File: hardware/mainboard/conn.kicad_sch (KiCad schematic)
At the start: 25 parts

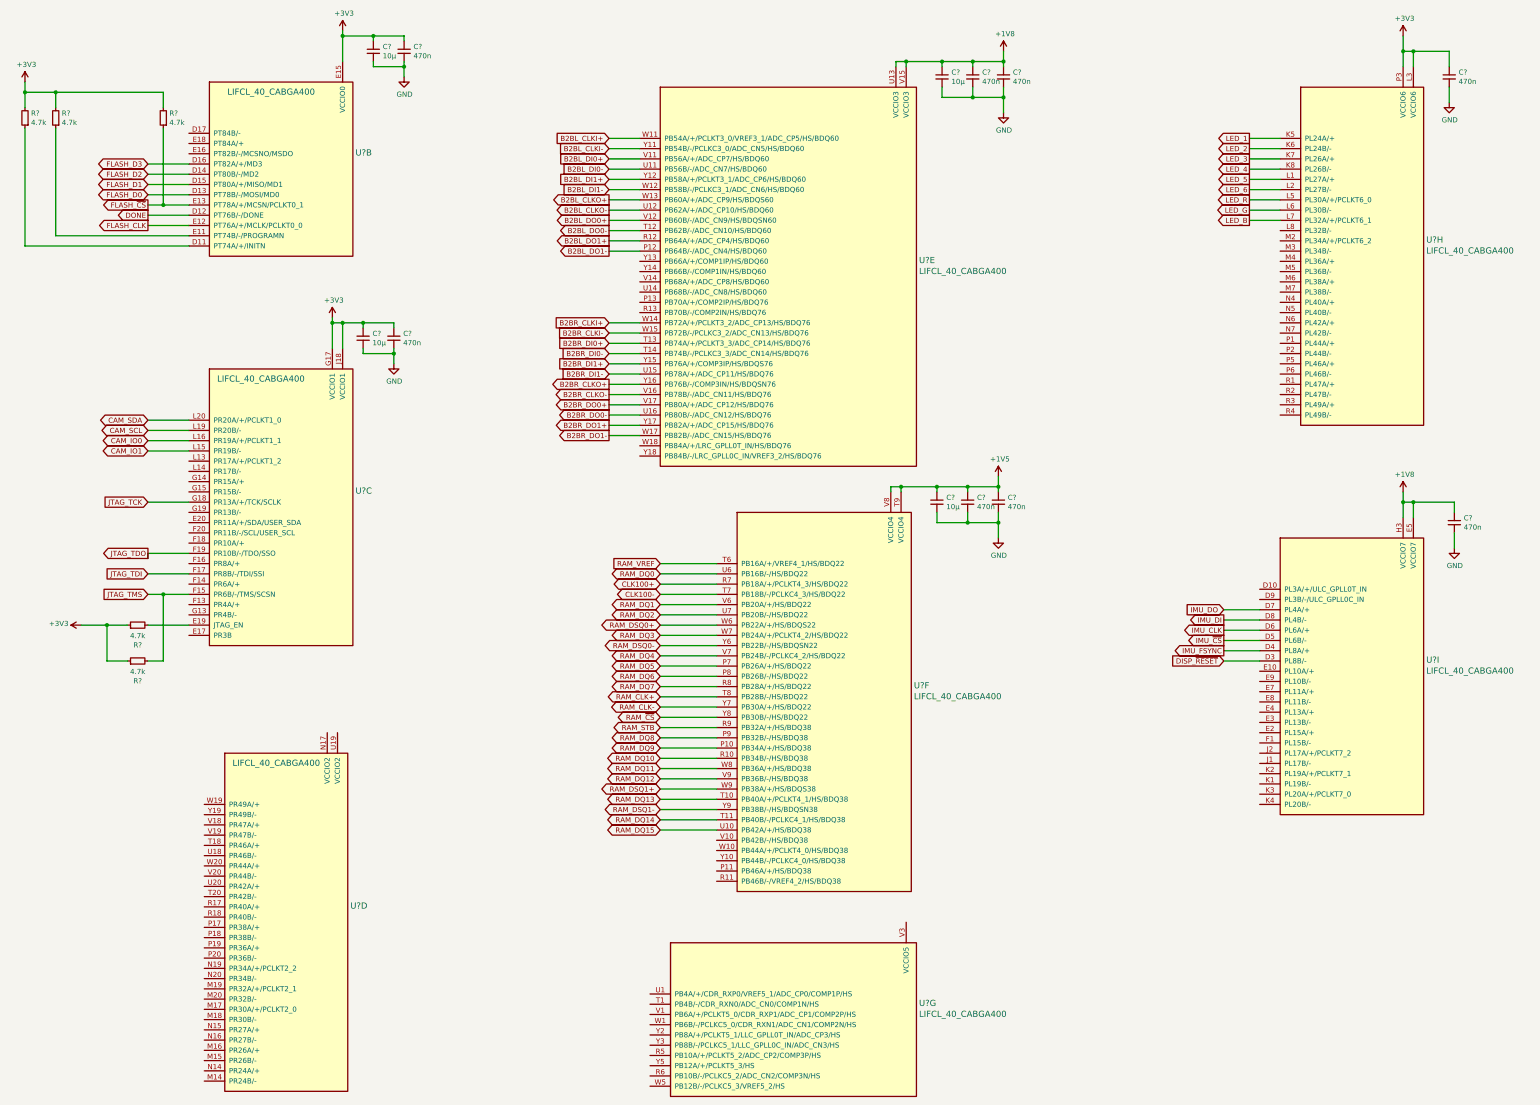
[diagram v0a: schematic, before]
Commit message: Connecting up various bits
Signed-off-by: David Shah <dave@ds0.me>
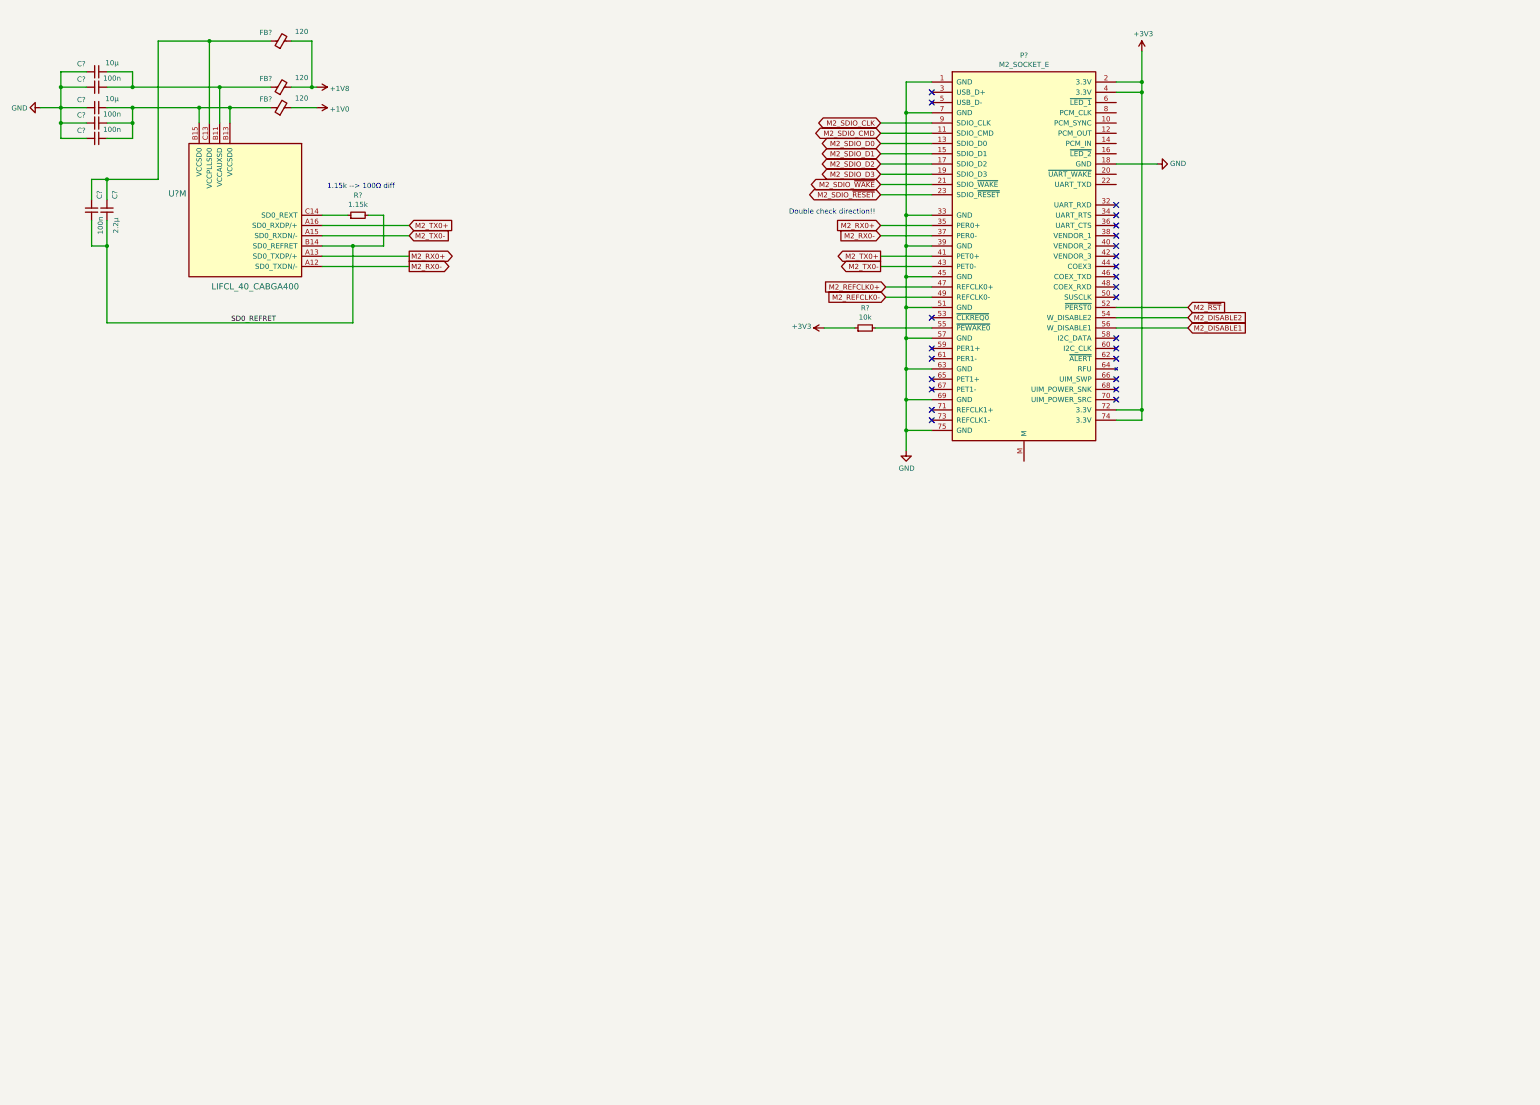
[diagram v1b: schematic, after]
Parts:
- removed C? (x4): 10µ, symbol Device:C_Small
- removed C? (x8): 470n, symbol Device:C_Small
- removed R? (x5): 4.7k, symbol Device:R_Small
- removed U? (x8): LIFCL_40_CABGA400, symbol meowality:LIFCL_40_CABGA400
- added C? (x4): 100n, symbol Device:C_Small
- added C? (x2): 10µ, symbol Device:C_Small
- added C?: 2.2µ, symbol Device:C_Small
- added FB? (x3): 120, symbol Device:FerriteBead_Small
- added P?: M2_SOCKET_E, symbol meowality:M2_SOCKET_E
- added R?: 1.15k, symbol Device:R_Small
- added R?: 10k, symbol Device:R_Small
- added U?: LIFCL_40_CABGA400, symbol meowality:LIFCL_40_CABGA400
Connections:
- net +1V8: now also FB?.2, FB?.2
- net +3V3: now also P?.2 (3.3V), P?.4 (3.3V), P?.72 (3.3V), P?.74 (3.3V), R?.1
- net GND: now also C?.2, C?.2, C?.2, C?.2, C?.2, P?.1 (GND), P?.18 (GND), P?.33 (GND), P?.39 (GND), P?.45 (GND), P?.51 (GND), P?.57 (GND), P?.63 (GND), P?.69 (GND), P?.7 (GND), P?.75 (GND)
- new net: C?.1, C?.1, C?.1, FB?.1, U?.B13 (VCCSD0), U?.B15 (VCCSD0)
- new net: C?.1, C?.1, FB?.1, U?.B11 (VCCAUXSD)
- new net: C?.2, C?.2, FB?.1, U?.C13 (VCCPLLSD0)
- new net: R?.1, U?.C14 (SD0_REXT)
- new net: P?.55 (~PEWAKE0), R?.2
- new net +1V0: FB?.2
- new net M2_DISABLE1: P?.56 (W_DISABLE1)
- new net M2_DISABLE2: P?.54 (W_DISABLE2)
- new net M2_REFCLK0+: P?.47 (REFCLK0+)
- new net M2_REFCLK0-: P?.49 (REFCLK0-)
- new net M2_RX0+: P?.35 (PER0+), U?.A13 (SD0_TXDP/+)
- new net M2_RX0-: P?.37 (PER0-), U?.A12 (SD0_TXDN/-)
- new net M2_SDIO_CLK: P?.9 (SDIO_CLK)
- new net M2_SDIO_CMD: P?.11 (SDIO_CMD)
- new net M2_SDIO_D0: P?.13 (SDIO_D0)
- new net M2_SDIO_D1: P?.15 (SDIO_D1)
- new net M2_SDIO_D2: P?.17 (SDIO_D2)
- new net M2_SDIO_D3: P?.19 (SDIO_D3)
- new net M2_SDIO_~RESET: P?.23 (SDIO_~RESET)
- new net M2_SDIO_~WAKE: P?.21 (SDIO_~WAKE)
- new net M2_TX0+: P?.41 (PET0+), U?.A16 (SD0_RXDP/+)
- new net M2_TX0-: P?.43 (PET0-), U?.A15 (SD0_RXDN/-)
- new net M2_~RST: P?.52 (~PERST0)
- new net SD0_REFRET: C?.1, C?.1, R?.2, U?.B14 (SD0_REFRET)
- no-connect marks 0 -> 25
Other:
- note added: "1.15k --> 100Ω diff"
- note added: "Double check direction!!"

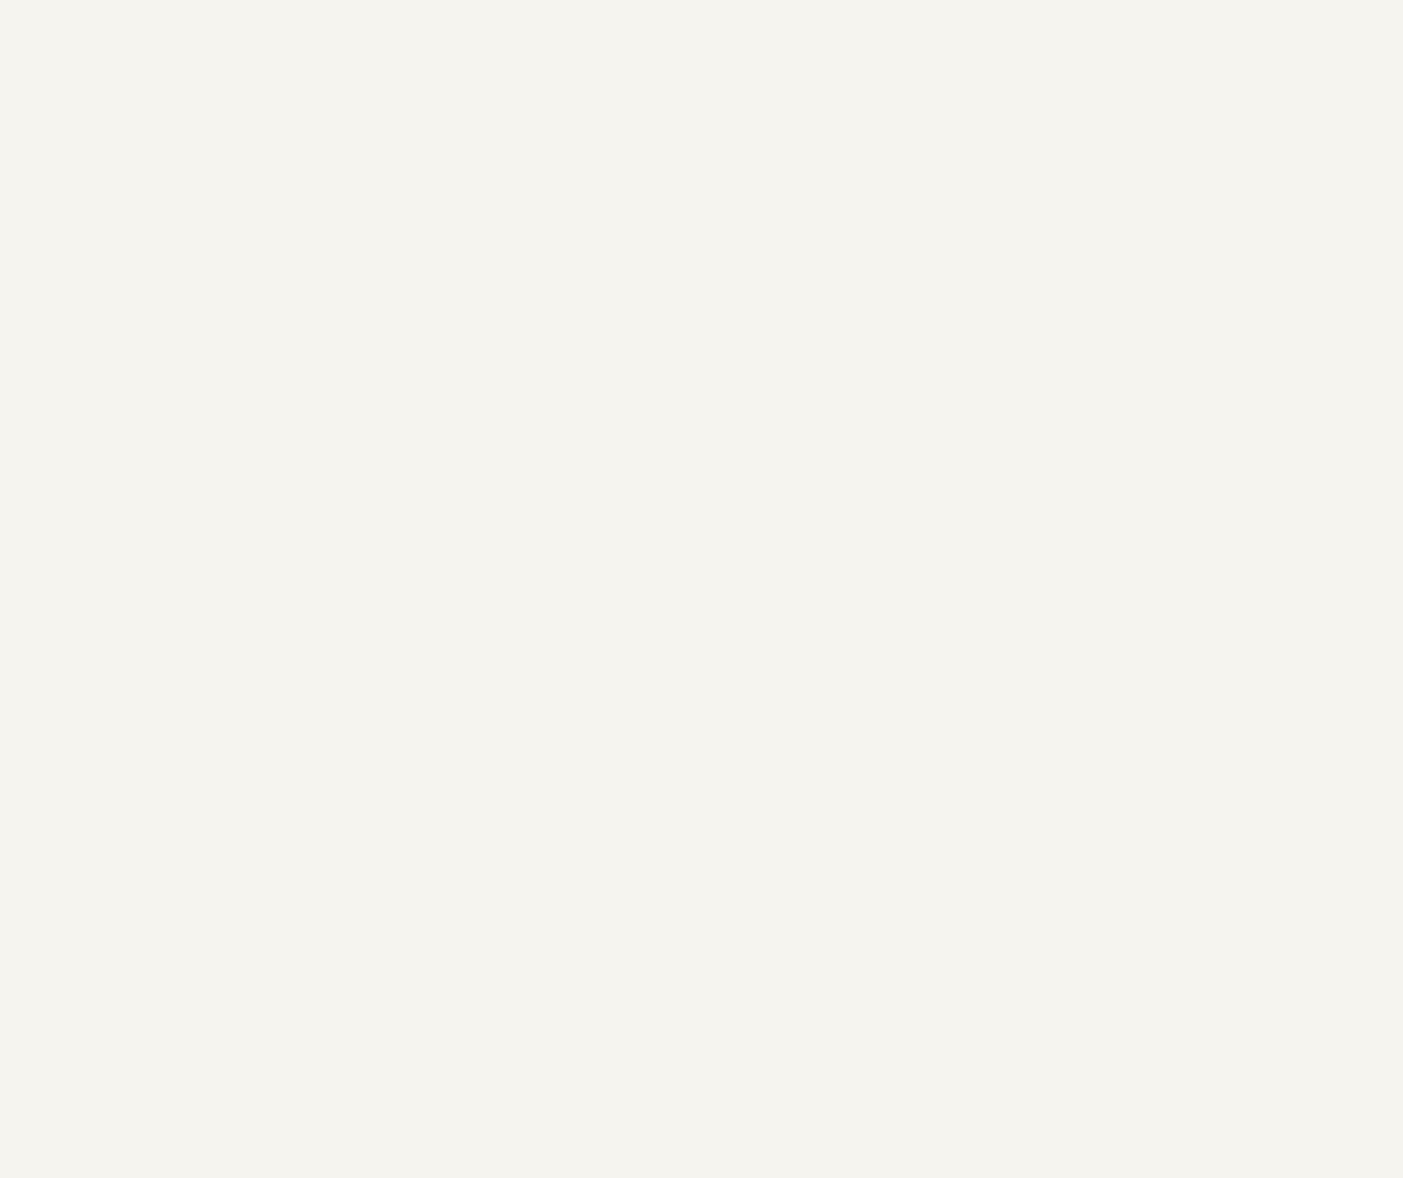
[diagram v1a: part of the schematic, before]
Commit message: Misc bits
Signed-off-by: David Shah <dave@ds0.me>
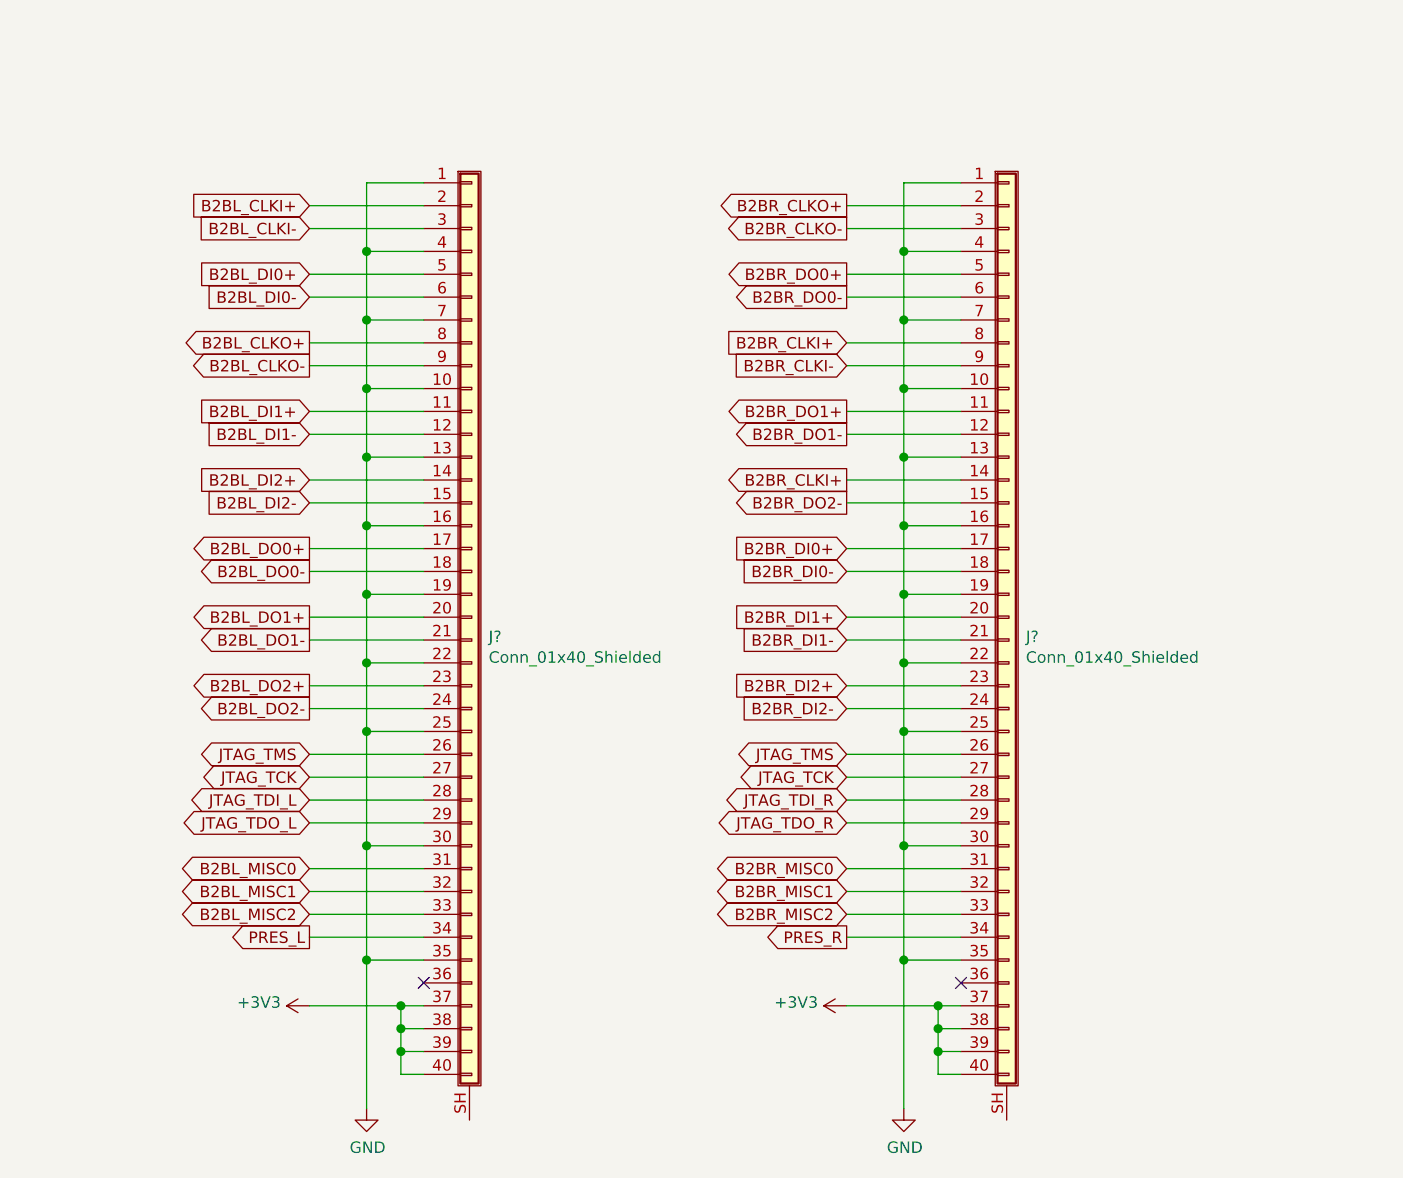
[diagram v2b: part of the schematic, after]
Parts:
- added J? (x2): Conn_01x40_Shielded, symbol Connector_Generic_Shielded:Conn_01x40_Shielded
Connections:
- net +3V3: now also J?.37 (Pin_37), J?.37 (Pin_37), J?.38 (Pin_38), J?.38 (Pin_38), J?.39 (Pin_39), J?.39 (Pin_39), J?.40 (Pin_40), J?.40 (Pin_40)
- net GND: now also J?.1 (Pin_1), J?.1 (Pin_1), J?.10 (Pin_10), J?.10 (Pin_10), J?.13 (Pin_13), J?.13 (Pin_13), J?.16 (Pin_16), J?.16 (Pin_16), J?.19 (Pin_19), J?.19 (Pin_19), J?.22 (Pin_22), J?.22 (Pin_22), J?.25 (Pin_25), J?.25 (Pin_25), J?.30 (Pin_30), J?.30 (Pin_30), J?.35 (Pin_35), J?.35 (Pin_35), J?.4 (Pin_4), J?.4 (Pin_4), J?.7 (Pin_7), J?.7 (Pin_7)
- new net B2BL_CLKI+: J?.2 (Pin_2)
- new net B2BL_CLKI-: J?.3 (Pin_3)
- new net B2BL_CLKO+: J?.8 (Pin_8)
- new net B2BL_CLKO-: J?.9 (Pin_9)
- new net B2BL_DI0+: J?.5 (Pin_5)
- new net B2BL_DI0-: J?.6 (Pin_6)
- new net B2BL_DI1+: J?.11 (Pin_11)
- new net B2BL_DI1-: J?.12 (Pin_12)
- new net B2BL_DI2+: J?.14 (Pin_14)
- new net B2BL_DI2-: J?.15 (Pin_15)
- new net B2BL_DO0+: J?.17 (Pin_17)
- new net B2BL_DO0-: J?.18 (Pin_18)
- new net B2BL_DO1+: J?.20 (Pin_20)
- new net B2BL_DO1-: J?.21 (Pin_21)
- new net B2BL_DO2+: J?.23 (Pin_23)
- new net B2BL_DO2-: J?.24 (Pin_24)
- new net B2BL_MISC0: J?.31 (Pin_31)
- new net B2BL_MISC1: J?.32 (Pin_32)
- new net B2BL_MISC2: J?.33 (Pin_33)
- new net B2BR_CLKI+: J?.14 (Pin_14), J?.8 (Pin_8)
- new net B2BR_CLKI-: J?.9 (Pin_9)
- new net B2BR_CLKO+: J?.2 (Pin_2)
- new net B2BR_CLKO-: J?.3 (Pin_3)
- new net B2BR_DI0+: J?.17 (Pin_17)
- new net B2BR_DI0-: J?.18 (Pin_18)
- new net B2BR_DI1+: J?.20 (Pin_20)
- new net B2BR_DI1-: J?.21 (Pin_21)
- new net B2BR_DI2+: J?.23 (Pin_23)
- new net B2BR_DI2-: J?.24 (Pin_24)
- new net B2BR_DO0+: J?.5 (Pin_5)
- new net B2BR_DO0-: J?.6 (Pin_6)
- new net B2BR_DO1+: J?.11 (Pin_11)
- new net B2BR_DO1-: J?.12 (Pin_12)
- new net B2BR_DO2-: J?.15 (Pin_15)
- new net B2BR_MISC0: J?.31 (Pin_31)
- new net B2BR_MISC1: J?.32 (Pin_32)
- new net B2BR_MISC2: J?.33 (Pin_33)
- new net JTAG_TCK: J?.27 (Pin_27), J?.27 (Pin_27)
- new net JTAG_TDI_L: J?.28 (Pin_28)
- new net JTAG_TDI_R: J?.28 (Pin_28)
- new net JTAG_TDO_L: J?.29 (Pin_29)
- new net JTAG_TDO_R: J?.29 (Pin_29)
- new net JTAG_TMS: J?.26 (Pin_26), J?.26 (Pin_26)
- new net PRES_L: J?.34 (Pin_34)
- new net PRES_R: J?.34 (Pin_34)
- no-connect marks 25 -> 27
